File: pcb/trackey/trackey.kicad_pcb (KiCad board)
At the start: 2 copper layers, 33 x 63.5 mm, 28 parts, among them J1 trackball_port, J10 is_left, J11 is_right, J12 is_left, J13 is_right, J14 OLED_conn, J2 RJ45, J3 COL_port, J4 ROW_port, J5 RJ45, J6 is_left, J7 is_right, J8 is_left, J9 is_right, U1 Arduino_Pro_Micro, U2 Arduino_Pro_Micro

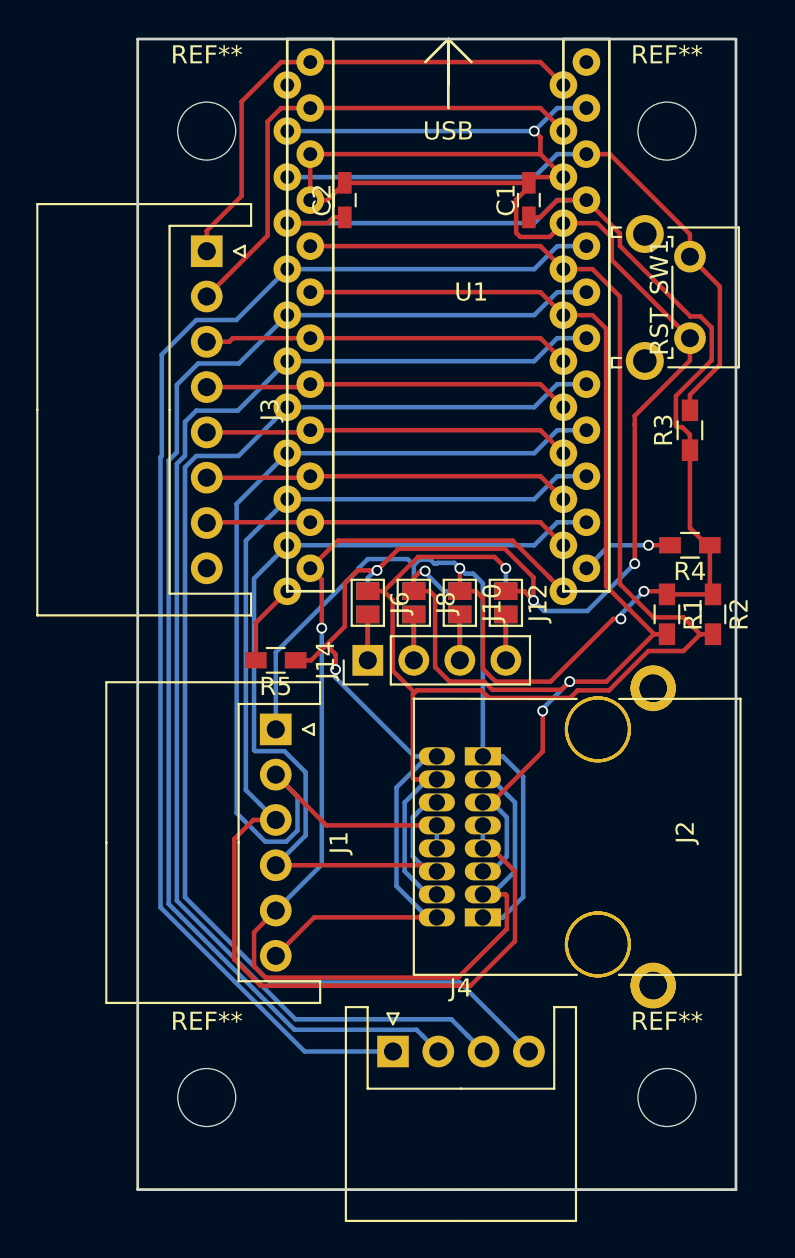
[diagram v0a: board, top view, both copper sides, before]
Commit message: improve trackey pcb
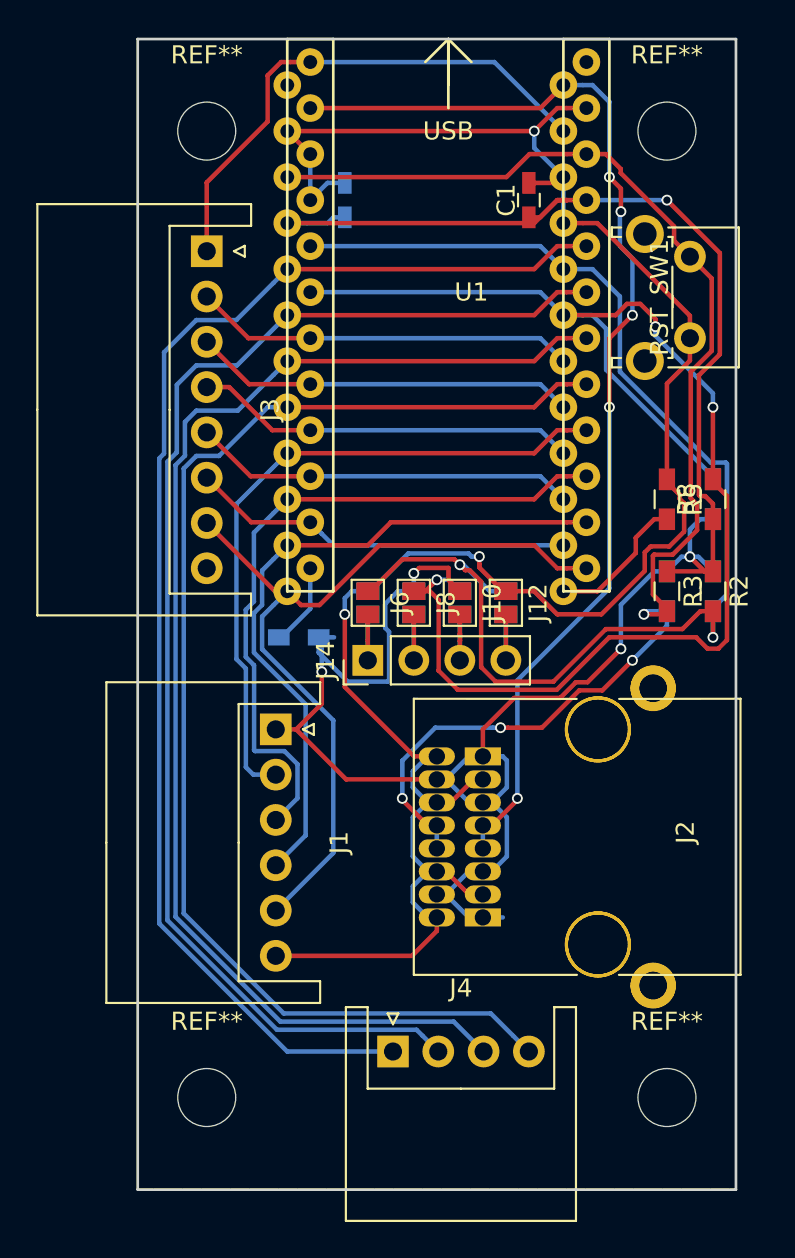
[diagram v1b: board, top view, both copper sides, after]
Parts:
- added R6: R, Resistors_SMD:R_0603_HandSoldering, B.Cu at (27.9, 25.4)
- added R7: R, Resistors_SMD:R_0603_HandSoldering, B.Cu at (27.9, 20.3)
- added R8: R, Resistors_SMD:R_0603_HandSoldering, F.Cu at (27.9, 20.3)
- C2, R4: moved to B.Cu
- R1: value 2.2k -> R; moved to B.Cu
- R2: value 2.2k -> R
- moved R5 23.3 mm to (25.4, 20.3), turned to 270 degrees
- moved R4 22.2 mm to (5.08, 27.9)
- moved R3 8.98 mm to (25.4, 25.4), turned to 270 degrees
- moved R1 1.27 mm to (25.4, 25.4)
- moved R2 1.27 mm to (27.9, 25.4)
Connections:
- net Net-(J3-Pad8) renamed /COL7
- J1 pad 5: /Trackball_SS -> /COL6
- J2 pad 2: /SDA -> +5V
- J2 pad 3: /SCL -> +5V
- J2 pad 4: /SCLK -> /RST
- J2 pad 5: /MISO -> /DATA
- J2 pad 6: /MOSI -> GND
- J2 pad 7: /Trackball_SS -> GND
- J5 pad 2: /SDA -> +5V
- J5 pad 3: /SCL -> +5V
- J5 pad 4: /SCLK -> /RST
- J5 pad 5: /MISO -> /DATA
- J5 pad 6: /MOSI -> GND
- J5 pad 7: /Trackball_SS -> GND
- R1 pad 2: /SCL -> /RST
- U1 pad 10: /COL5 -> /COL4
- U1 pad 11: /COL6 -> /COL5
- U1 pad 12: /Trackball_SS -> Net-(R4-Pad2)
- U1 pad 13: Net-(R4-Pad2) -> /COL6
- U1 pad 2: /COL1 -> /DATA
- U1 pad 7: /COL2 -> /COL1
- U1 pad 8: /COL3 -> /COL2
- U1 pad 9: /COL4 -> /COL3
- U2 pad 1: /COL0 -> /DATA
- U2 pad 10: /COL5 -> /COL4
- U2 pad 11: /COL6 -> /COL5
- U2 pad 12: /Trackball_SS -> Net-(R5-Pad2)
- U2 pad 13: Net-(R5-Pad2) -> /COL6
- U2 pad 2: /COL1 -> /COL0
- U2 pad 7: /COL2 -> /COL1
- U2 pad 8: /COL3 -> /COL2
- U2 pad 9: /COL4 -> /COL3
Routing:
- net /Trackball_SS: track 66.5 -> 0.00 mm, vias 1 -> 0
- net /DATA: track 0.00 -> 62.9 mm, vias 0 -> 5
- net /RST: track 35.7 -> 75.4 mm, vias 0 -> 4
- net /MISO: track 70.3 -> 38.3 mm
- net /COL6: track 20.2 -> 45.9 mm
- net GND: track 139.8 -> 118.2 mm, vias 5 -> 3
- net /SCLK: track 57.2 -> 37.6 mm
- net +5V: track 114.4 -> 131.8 mm, vias 3 -> 5
- net /SDA: track 88.6 -> 71.8 mm, vias 1 -> 2
- net /MOSI: track 52.8 -> 37.3 mm
- net /COL1: track 28.2 -> 21.2 mm
- net /SCL: track 73.3 -> 79.5 mm
- net Net-(R5-Pad2): track 4.53 -> 7.86 mm
- net /COL0: track 28.2 -> 29.3 mm
- net /COL5: track 20.2 -> 21.2 mm
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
